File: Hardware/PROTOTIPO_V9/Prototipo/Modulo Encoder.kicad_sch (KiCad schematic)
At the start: 3 parts, among them J5 Conn_01x05, J6 Conn_01x05, U7 KY-040

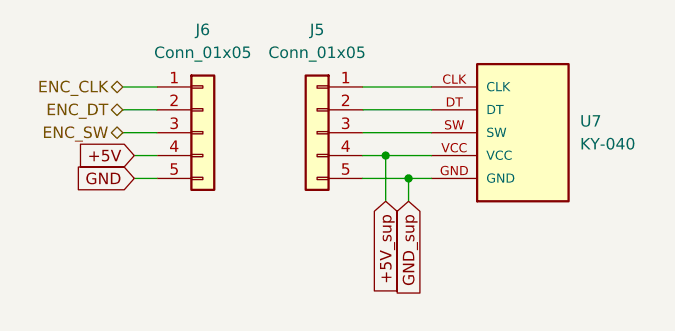
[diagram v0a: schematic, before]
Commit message: Bus de salida
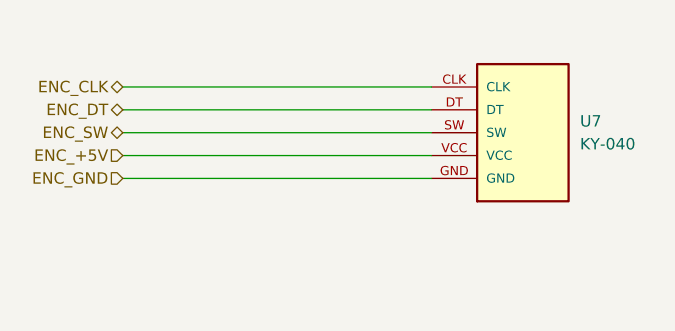
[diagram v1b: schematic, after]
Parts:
- removed J5, J6: Conn_01x05, symbol Connector_Generic:Conn_01x05
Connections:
- net ENC_CLK: now also U7.CLK
- net ENC_DT: now also U7.DT
- net ENC_SW: now also U7.SW
- net +5V_sup renamed ENC_+5V
- net GND_sup renamed ENC_GND
